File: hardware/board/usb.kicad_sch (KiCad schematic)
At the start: 0 parts

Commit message: emmc stuff
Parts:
- added C118, C119: 100nF X5R 10V, Capacitor_SMD:C_0201_0603Metric, symbol Device:C
- added C120: 1uF X5R 10V, Capacitor_SMD:C_0402_1005Metric, symbol Device:C
- added C121: 100nF X5R 10V, Capacitor_SMD:C_0402_1005Metric, symbol Device:C
- added C122: 120uF SVPF 20V, Capacitor_SMD:CP_Elec_6.3x5.9, symbol Device:C_Polarized
- added D10, D11: BZT52C5V1_C173407, lcsc:SOD-123_L2.7-W1.6-LS3.7-RD, symbol lcsc:BZT52C5V1_C173407
- added J3: USB3_A, symbol Connector:USB3_A
- added L10: L_Iron_Coupled_Small, lcsc:FILTER-SMD_4P-L2.0-W1.2-BL_DLW21H, symbol Device:L_Iron_Coupled_Small
- added R58, R59: 0R 5%, Resistor_SMD:R_0201_0603Metric, symbol Device:R
- added R62, R63: 0R 5%, Resistor_SMD:R_0402_1005Metric, symbol Device:R
- added R64, R65: 2.2R 5%, Resistor_SMD:R_0402_1005Metric, symbol Device:R
- added R66: 4.7K 5%, Resistor_SMD:R_0402_1005Metric, symbol Device:R
- added U14, U15, U16, U17: ESD5311X, lcsc:DFN1006-2L-BI, symbol lcsc:ESD5311X_C2844730
- added U18: SY6280AAC, lcsc:SOT-23-5_L3.0-W1.7-P0.95-LS2.8-BL, symbol lcsc:SY6280AAC
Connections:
- new net: C118.1, J3.9 (SSTX+), U15.2
- new net: L10.3, R63.1, R65.1
- new net: L10.1, R62.2, R64.1
- new net: C119.1, J3.8 (SSTX-), U14.2
- new net: J3.6 (SSRX+), R58.1, U17.2
- new net: J3.5 (SSRX-), R59.1, U16.2
- new net: R66.1, U18.3 (ISET)
- new net GND: C120.1, C121.2, C122.2, D10.2 (A), D11.2 (A), J3.10 (SHIELD), J3.4 (GND), J3.7 (DRAIN), R66.2, U14.1, U15.1, U16.1, U17.1, U18.2 (GND)
- new net USB3_HOST1DM: D11.1 (C), J3.2 (D-), L10.4, R63.2
- new net USB3_HOST1DP: D10.1 (C), J3.3 (D+), L10.2, R62.1
- new net USB3_HOST1_SSRXN: R59.2
- new net USB3_HOST1_SSRXP: R58.2
- new net USB3_HOST1_SSTXN: C119.2
- new net USB3_HOST1_SSTXP: C118.2
- new net USB3_OTG0_DM: R65.2
- new net USB3_OTG0_DP: R64.2
- new net USB_HOST_PWREN_H_GPIO0_A6: U18.4 (EN)
- new net VCC5V0_USB_HOST1: C121.1, C122.1, J3.1 (VBUS), U18.1 (OUT)
- new net VCC_5V0: C120.2, U18.5 (IN)

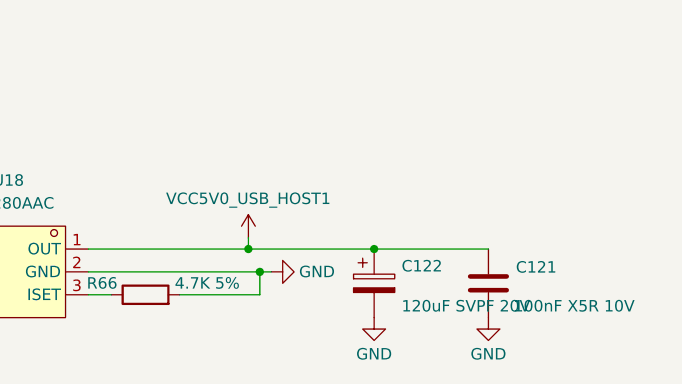
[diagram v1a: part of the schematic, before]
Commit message: start of ethernet
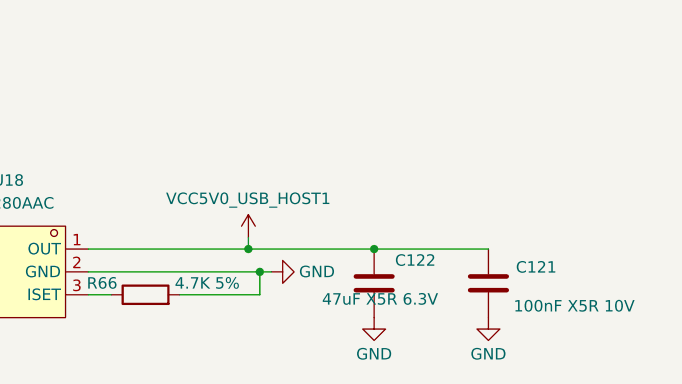
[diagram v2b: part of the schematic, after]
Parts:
- removed C122: 120uF SVPF 20V, Capacitor_SMD:CP_Elec_6.3x5.9, symbol Device:C_Polarized
- added C122: 47uF X5R 6.3V, Capacitor_SMD:C_0805_2012Metric, symbol Device:C
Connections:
- net GND: now also C122.1
- net VCC5V0_USB_HOST1: now also C122.2
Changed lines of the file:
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@@
+	)
+	(junction
+		(at 82.55 97.79)
+		(diameter 0)
+		(color 0 0 0 0)
+	)
+	(junction
+		(at 82.55 100.33)
+		(diameter 0)
+		(color 0 0 0 0)
+	)
+	(junction
+		(at 78.74 54.61)
+		(diameter 0)
+		(color 0 0 0 0)
+	)
+	(junction
+		(at 60.96 46.99)
+		(diameter 0)
+		(color 0 0 0 0)
+	)
+	(junction
+		(at 72.39 100.33)
+		(diameter 0)
+		(color 0 0 0 0)
 	)
 	(junction
@@
 	)
 	(junction
-		(at 82.55 97.79)
-		(diameter 0)
-		(color 0 0 0 0)
-	)
-	(junction
-		(at 82.55 100.33)
-		(diameter 0)
-		(color 0 0 0 0)
-	)
-	(junction
-		(at 78.74 54.61)
-		(diameter 0)
-		(color 0 0 0 0)
-	)
-	(junction
-		(at 60.96 46.99)
-		(diameter 0)
-		(color 0 0 0 0)
-	)
-	(junction
-		(at 72.39 100.33)
-		(diameter 0)
-		(color 0 0 0 0)
-	)
-	(junction
 		(at 74.93 100.33)
 		(diameter 0)
@@
 	(wire
 		(pts
-			(xy 214.63 107.95) (xy 200.66 107.95)
+			(xy 200.66 107.95) (xy 214.63 107.95)
 		)
 		(stroke
@@
 	(wire
 		(pts
+			(xy 214.63 107.95) (xy 227.33 107.95)
+		)
+		(stroke
+			(width 0)
+			(type default)
+		)
+	)
+	(wire
+		(pts
 			(xy 43.18 62.23) (xy 43.18 63.5)
 		)
@@
 		(pts
 			(xy 201.93 113.03) (xy 201.93 110.49)
-		)
-		(stroke
-			(width 0)
-			(type default)
-		)
-	)
-	(wire
-		(pts
-			(xy 214.63 107.95) (xy 227.33 107.95)
 		)
 		(stroke
@@
 	)
 	(symbol
-		(lib_id "Device:C_Polarized")
-		(at 214.63 111.76 0)
-		(unit 1)
-		(exclude_from_sim no)
-		(in_bom yes)
-		(on_board yes)
-		(dnp no)
-		(property "Reference" "C122"
-			(at 217.678 109.8549 0)
-			(effects
-				(font
-					(size 1.27 1.27)
-				)
-				(justify left)
-			)
-		)
-		(property "Value" "120uF\nSVPF\n20V"
-			(at 217.678 114.3 0)
-			(effects
-				(font
-					(size 1.27 1.27)
-				)
-				(justify left)
-			)
-		)
-		(property "Footprint" "Capacitor_SMD:CP_Elec_6.3x5.9"
-			(at 215.5952 115.57 0)
-			(effects
-				(font
-					(size 1.27 1.27)
-				)
-				(hide yes)
-			)
-		)
-		(property "Datasheet" "~"
-			(at 214.63 111.76 0)
-			(effects
-				(font
-					(size 1.27 1.27)
-				)
-				(hide yes)
-			)
-		)
-		(property "Description" "Polarized capacitor"
-			(at 214.63 111.76 0)
-			(effects
-				(font
-					(size 1.27 1.27)
-				)
-				(hide yes)
-			)
-		)
-		(property "LCSC" "C371973"
-			(at 214.63 111.76 0)
-			(effects
-				(font
-					(size 1.27 1.27)
-				)
-				(hide yes)
-			)
-		)
-		(pin "1"
-		)
-		(pin "2"
-		)
-		(instances
-			(project ""
-				(path "/3bc38516-4fe0-4022-adb8-9fd55b66cd2d/c07c3c7a-b8b0-4fa9-bbf1-2e0263ea0c12"
-					(reference "C122")
-					(unit 1)
-				)
-			)
-		)
-	)
-	(symbol
 		(lib_id "power:GND")
 		(at 66.04 113.03 0)
@@
 					(unit 1)
 				)
+			)
+		)
+	)
+	(symbol
+		(lib_id "Device:C")
+		(at 214.63 111.76 0)
+		(mirror x)
+		(unit 1)
+		(exclude_from_sim no)
+		(in_bom yes)
+		(on_board yes)
+		(dnp no)
+		(property "Reference" "C122"
+			(at 221.488 109.22 0)
+			(effects
+				(font
+					(size 1.27 1.27)
+				)
+				(justify right)
+			)
+		)
+		(property "Value" "47uF\nX5R\n6.3V"
+			(at 221.742 113.538 0)
+			(effects
+				(font
+					(size 1.27 1.27)
+				)
+				(justify right)
+			)
+		)
+		(property "Footprint" "Capacitor_SMD:C_0805_2012Metric"
+			(at 215.5952 107.95 0)
+			(effects
+				(font
+					(size 1.27 1.27)
+				)
+				(hide yes)
+			)
+		)
+		(property "Datasheet" "~"
+			(at 214.63 111.76 0)
+			(effects
+				(font
+					(size 1.27 1.27)
+				)
+				(hide yes)
+			)
+		)
+		(property "Description" "Unpolarized capacitor"
+			(at 214.63 111.76 0)
+			(effects
+				(font
+					(size 1.27 1.27)
+				)
+				(hide yes)
+			)
+		)
+		(pin "2"
+		)
+		(pin "1"
+		)
+		(instances
+			(project "frost"
+				(path "/3bc38516-4fe0-4022-adb8-9fd55b66cd2d/c07c3c7a-b8b0-4fa9-bbf1-2e0263ea0c12"
+					(reference "C122")
+					(unit 1)
+				)

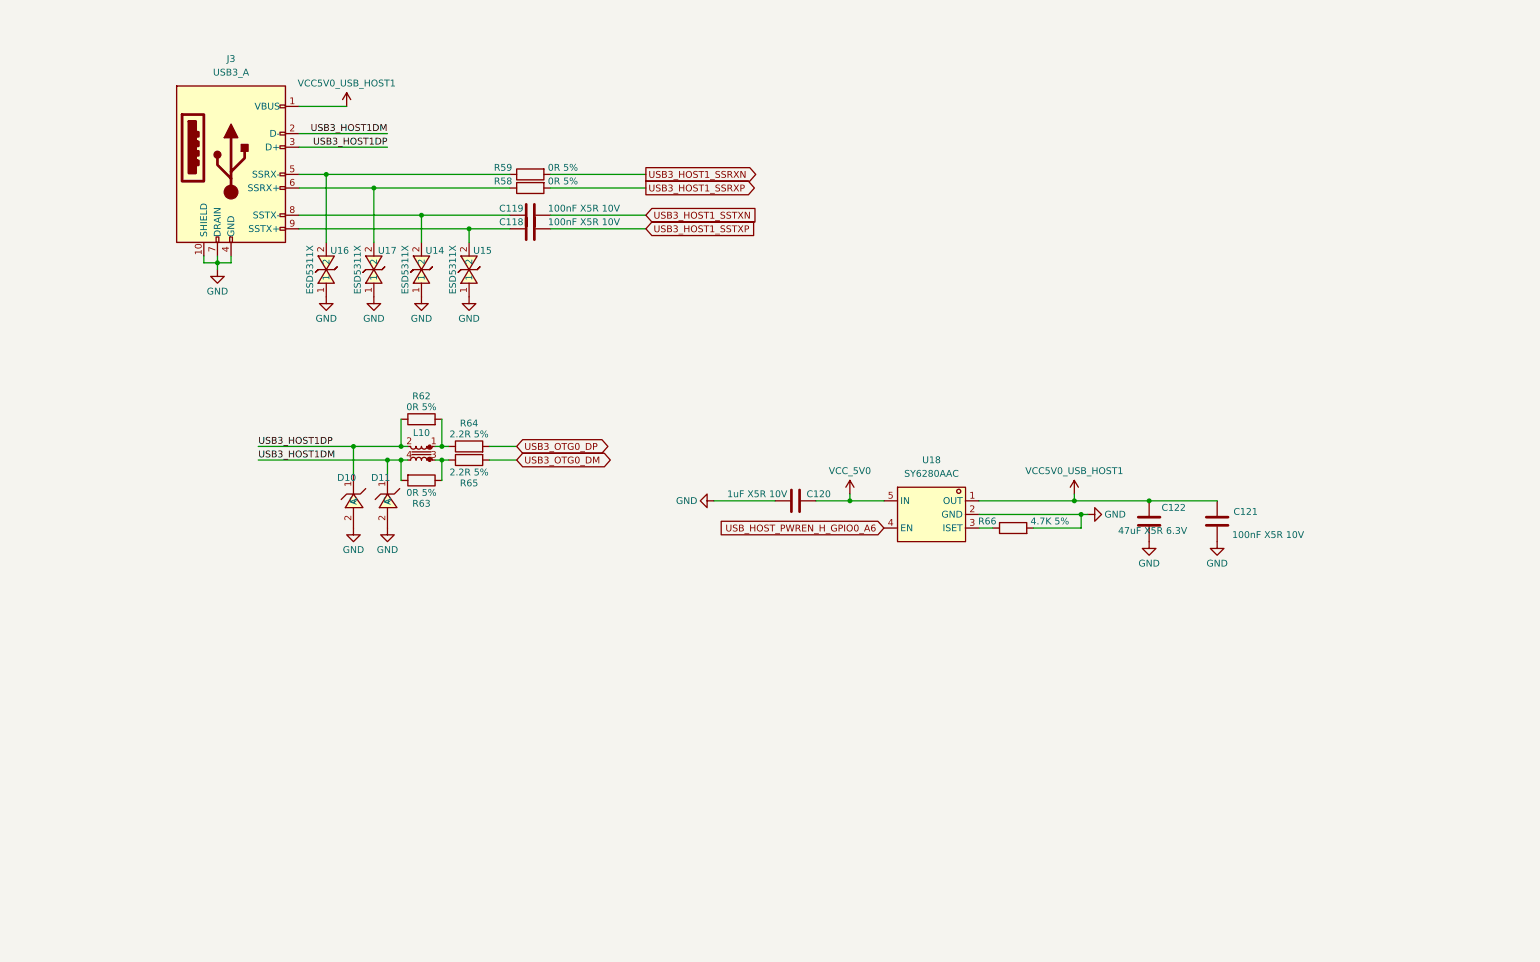
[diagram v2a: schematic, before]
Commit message: finished schematic!
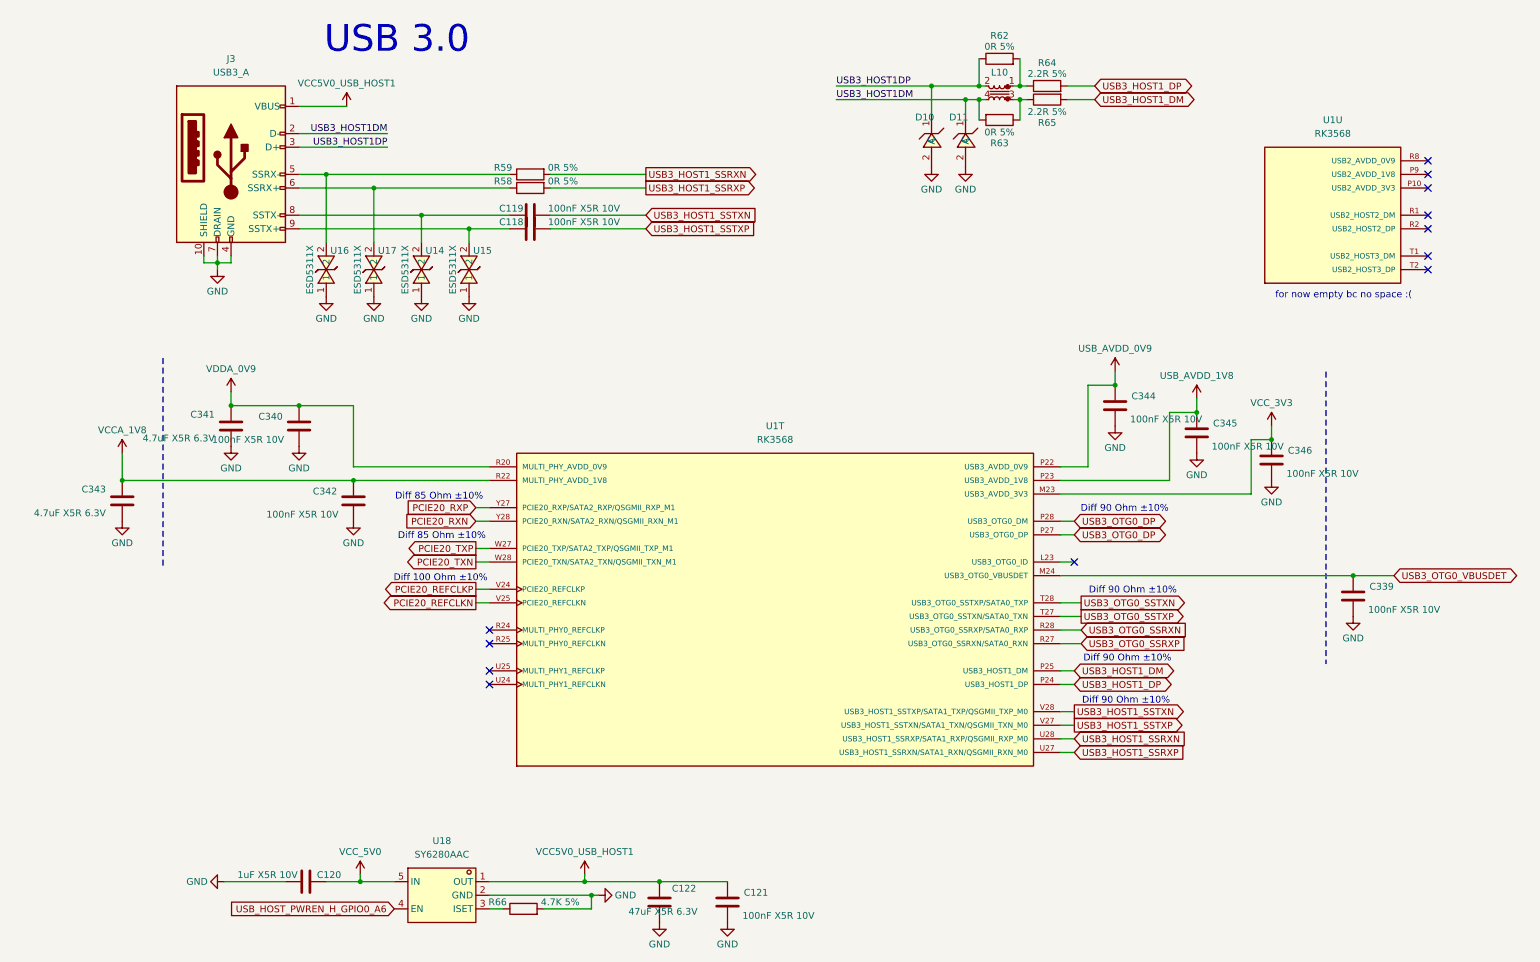
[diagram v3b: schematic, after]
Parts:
- added C339: 100nF X5R 10V, Capacitor_SMD:C_0402_1005Metric, symbol Device:C
- added C340, C342, C344, C345, C346: 100nF X5R 10V, Capacitor_SMD:C_0201_0603Metric, symbol Device:C
- added C341, C343: 4.7uF X5R 6.3V, Capacitor_SMD:C_0402_1005Metric, symbol Device:C
- added U1: RK3568, RK3568:BGA636C65P28X28_1900X1900X168, symbol RK3568:RK3568
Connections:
- net GND: now also C339.2, C340.2, C341.2, C342.2, C343.2, C344.2, C345.2, C346.2
- net USB3_HOST1_SSRXN: now also U1.U28 (USB3_HOST1_SSRXP/SATA1_RXP/QSGMII_RXP_M0)
- net USB3_HOST1_SSRXP: now also U1.U27 (USB3_HOST1_SSRXN/SATA1_RXN/QSGMII_RXN_M0)
- net USB3_HOST1_SSTXN: now also U1.V28 (USB3_HOST1_SSTXP/SATA1_TXP/QSGMII_TXP_M0)
- net USB3_HOST1_SSTXP: now also U1.V27 (USB3_HOST1_SSTXN/SATA1_TXN/QSGMII_TXN_M0)
- net USB3_OTG0_DP: now also U1.P27 (USB3_OTG0_DP), U1.P28 (USB3_OTG0_DM); no longer R64.2
- net USB3_OTG0_DM renamed USB3_HOST1_DM
- net USB3_HOST1_DM: now also U1.P25 (USB3_HOST1_DM)
- new net MULTI_PHY_AVDD_0V9: C340.1, C341.1, U1.R20 (MULTI_PHY_AVDD_0V9), U1.R21 (MULTI_PHY_AVDD_0V9)
- new net PCIE20_REFCLKN: U1.V25 (PCIE20_REFCLKN)
- new net PCIE20_REFCLKP: U1.V24 (PCIE20_REFCLKP)
- new net PCIE20_RXN: U1.Y28 (PCIE20_RXN/SATA2_RXN/QSGMII_RXN_M1)
- new net PCIE20_RXP: U1.Y27 (PCIE20_RXP/SATA2_RXP/QSGMII_RXP_M1)
- new net PCIE20_TXN: U1.W28 (PCIE20_TXN/SATA2_TXN/QSGMII_TXN_M1)
- new net PCIE20_TXP: U1.W27 (PCIE20_TXP/SATA2_TXP/QSGMII_TXP_M1)
- new net USB3_HOST1_DP: R64.2, U1.P24 (USB3_HOST1_DP)
- new net USB3_OTG0_SSRXN: U1.R28 (USB3_OTG0_SSRXP/SATA0_RXP)
- new net USB3_OTG0_SSRXP: U1.R27 (USB3_OTG0_SSRXN/SATA0_RXN)
- new net USB3_OTG0_SSTXN: U1.T28 (USB3_OTG0_SSTXP/SATA0_TXP)
- new net USB3_OTG0_SSTXP: U1.T27 (USB3_OTG0_SSTXN/SATA0_TXN)
- new net USB3_OTG0_VBUSDET: C339.1, U1.M24 (USB3_OTG0_VBUSDET)
- new net USB_AVDD_0V9: C344.1, U1.P22 (USB3_AVDD_0V9)
- new net USB_AVDD_1V8: C345.1, U1.P23 (USB3_AVDD_1V8)
- new net VCCA_1V8: C342.1, C343.1, U1.R22 (MULTI_PHY_AVDD_1V8)
- new net VCC_3V3: C346.1, U1.M23 (USB3_AVDD_3V3)
- no-connect marks 0 -> 12
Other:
- note added: "Diff 100 Ohm ±10%"
- note added: "Diff 85 Ohm ±10%"
- note added: "Diff 90 Ohm ±10%"
- note added: "USB 3.0"
- note added: "for now empty bc no space :("
- moved on the sheet: C120, C121, C122, D10, D11, L10, R62, R63, R64, R65, R66, U18
